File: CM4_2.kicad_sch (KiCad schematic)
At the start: 22 parts, among them J1 Bus_PCI_Express_Mini, J10 PCIE_USB_D-/D+, J11 V_IN1, J12 V_IN2, J17 GPIO_V, J2 USB_A, J20 Controll Connector, J3 USB_HUB, J30 GPIO Connector, J4 USB_B_Micro, J40 N_LED, J41 GND, J42 1V5, J5 Micro_SD_Card, J6 HDMI_A_1.4, J7 USB_OTG, J9 RJ45

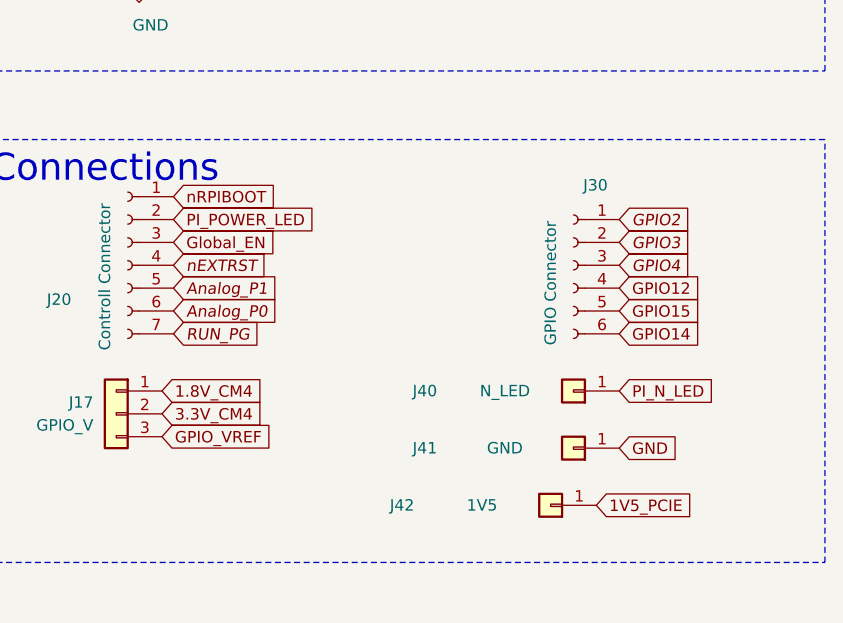
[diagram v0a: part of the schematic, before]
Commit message: v1.01
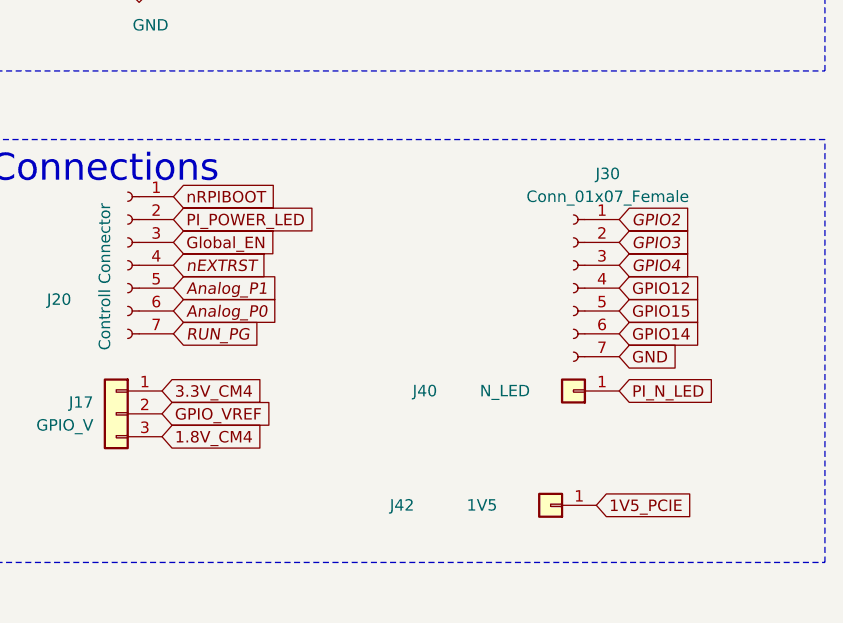
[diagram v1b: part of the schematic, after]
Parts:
- removed J30: GPIO Connector, Connector_PinHeader_2.54mm:PinHeader_1x06_P2.54mm_Vertical, symbol Connector:Conn_01x06_Female
- removed J41: GND, Connector_PinHeader_2.54mm:PinHeader_1x01_P2.54mm_Vertical, symbol Connector_Generic:Conn_01x01
- added J30: Conn_01x07_Female, Connector_PinSocket_2.54mm:PinSocket_1x07_P2.54mm_Vertical, symbol Connector:Conn_01x07_Female
- J17: footprint Connector_PinHeader_2.54mm:PinHeader_1x03_P2.54mm_Vertical -> Connector_PinHeader_2.54mm:PinHeader_1x03_P2.54mm_Vertical_SMD_Pin1Right
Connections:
- net 1.8V_CM4: now also J17.3 (Pin_3); no longer J17.1 (Pin_1)
- net 3.3V_CM4: now also J17.1 (Pin_1); no longer J17.2 (Pin_2)
- net GND: now also J30.7 (Pin_7)
- net GPIO12: now also J30.4 (Pin_4)
- net GPIO14: now also J30.6 (Pin_6)
- net GPIO15: now also J30.5 (Pin_5)
- net GPIO2: now also J30.1 (Pin_1)
- net GPIO3: now also J30.2 (Pin_2)
- net GPIO4: now also J30.3 (Pin_3)
- net GPIO_VREF: now also J17.2 (Pin_2); no longer J17.3 (Pin_3)
